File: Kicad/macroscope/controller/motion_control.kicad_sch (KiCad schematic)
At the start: 19 parts, among them J3 X stepper, J4 Y stepper, J5 Probe coil, M1 Stepper, M3 Stepper, U2 Coil driver

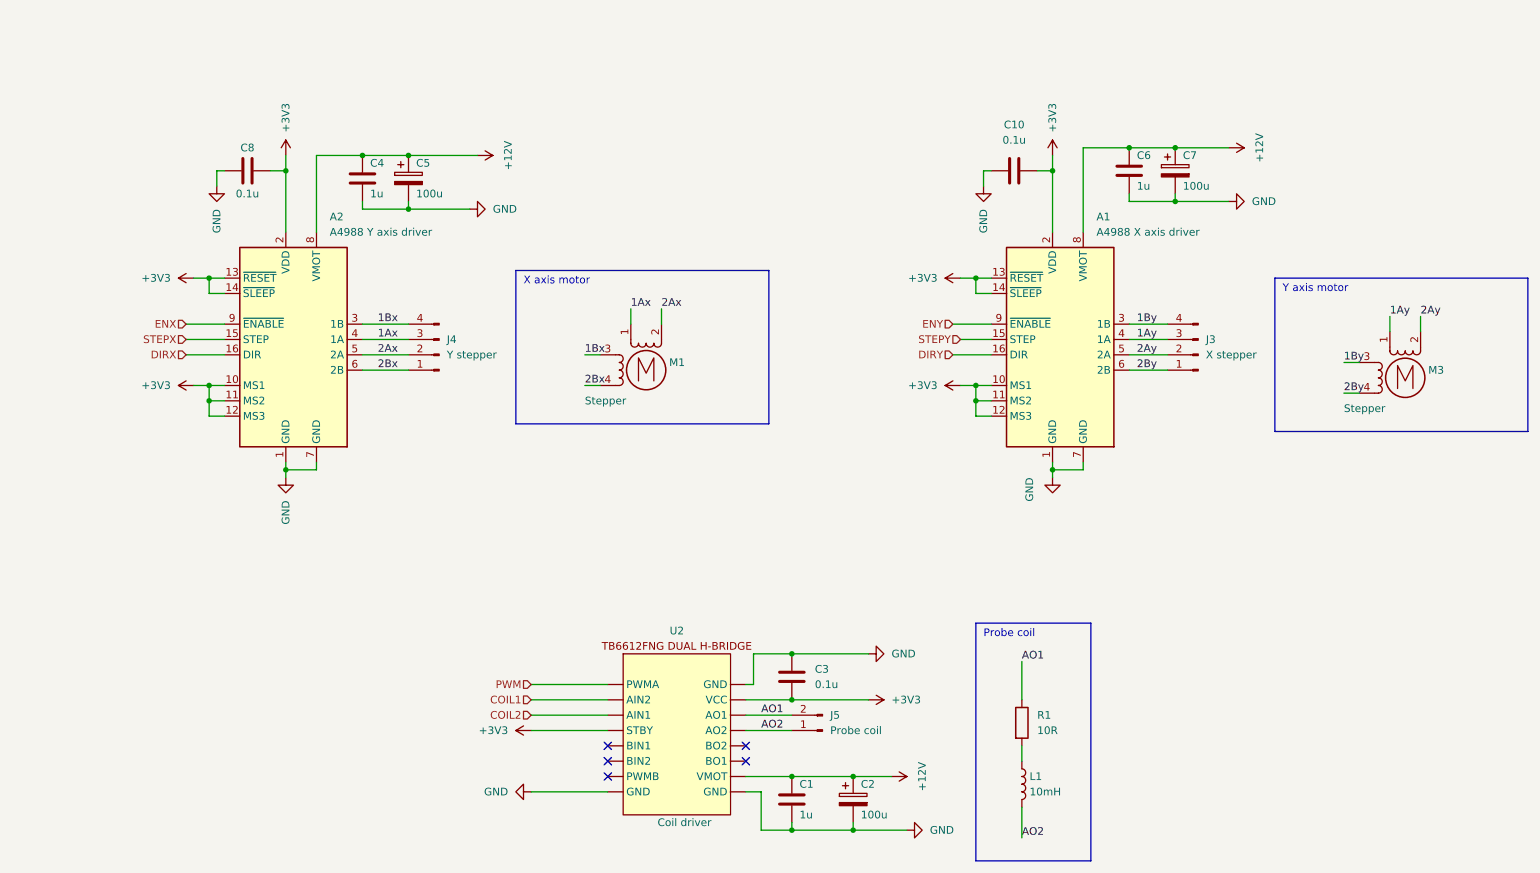
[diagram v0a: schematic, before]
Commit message: Update Kicad files
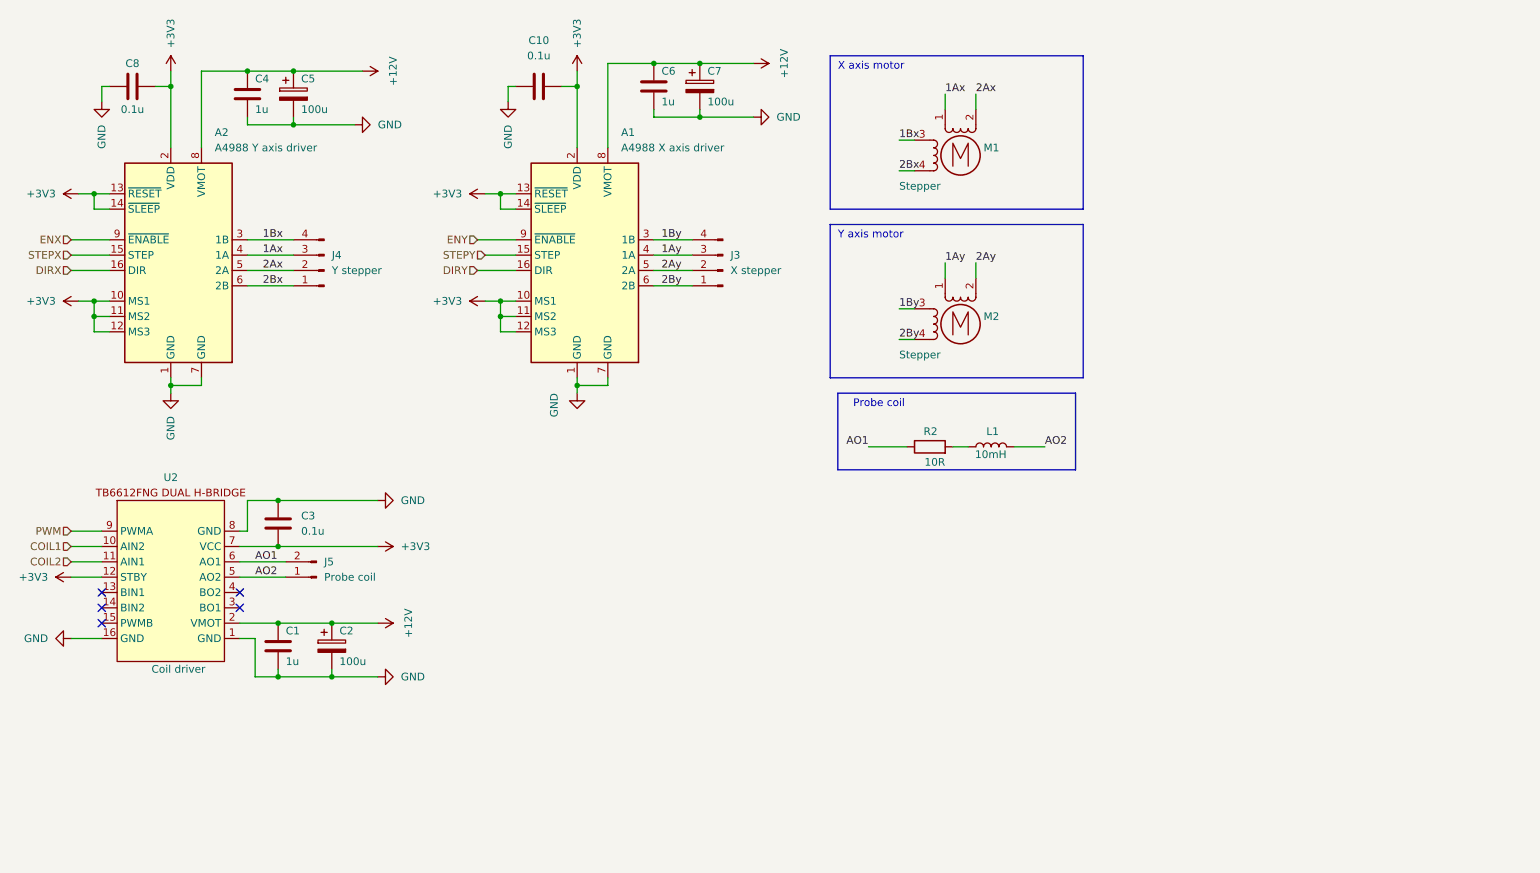
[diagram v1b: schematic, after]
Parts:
- C1, C10, C3, C4, C6, C8: footprint (none) -> Capacitor_SMD:C_1206_3216Metric
- C2, C5, C7: footprint (none) -> Capacitor_THT:CP_Radial_D6.3mm_P2.50mm
- J3, J4: footprint (none) -> Connector_PinHeader_2.54mm:PinHeader_1x04_P2.54mm_Vertical
- J5: footprint (none) -> Connector_Molex:Molex_KK-254_AE-6410-02A_1x02_P2.54mm_Vertical
- U2: footprint (none) -> Module:Pololu_Breakout-16_15.2x20.3mm
- renumbered M3 to M2, R1 to R2
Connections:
- net +12V: now also U2.2 (VMOT); no longer U2. (VMOT)
- net +3V3: now also U2.12 (STBY), U2.7 (VCC); no longer U2. (VMOT)
- net AO1: now also U2.6 (AO1); no longer U2. (VMOT)
- net AO2: now also U2.5 (AO2); no longer U2. (VMOT)
- net COIL1: now also U2.10 (AIN2); no longer U2. (VMOT)
- net COIL2: now also U2.11 (AIN1); no longer U2. (VMOT)
- net GND: now also U2.1 (GND), U2.16 (GND), U2.8 (GND); no longer U2. (VMOT)
- net PWM: now also U2.9 (PWMA); no longer U2. (VMOT)
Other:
- moved on the sheet: A1, A2, C1, C10, C2, C3, C4, C5, C6, C7, C8, J3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

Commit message: Add CAD
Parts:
- A1, A2: footprint Module:Pololu_Breakout-16_15.2x20.3mm -> Custom footprints:A4988_Pololu_Breakout-16_15.2x20.3mm
- U2: footprint Module:Pololu_Breakout-16_15.2x20.3mm -> Custom footprints:TB6612FNG_Pololu_Breakout-16_15.2x20.3mm
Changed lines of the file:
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@@
       (effects (font (size 1.27 1.27)))
     )
-    (property "Footprint" "Module:Pololu_Breakout-16_15.2x20.3mm" (at 41.91 106.68 0)
+    (property "Footprint" "Custom footprints:TB6612FNG_Pololu_Breakout-16_15.2x20.3mm" (at 41.91 106.68 0)
       (effects (font (size 1.27 1.27)) hide)
     )
@@
       (effects (font (size 1.27 1.27)) (justify left))
     )
-    (property "Footprint" "Module:Pololu_Breakout-16_15.2x20.3mm" (at 116.205 72.39 0)
+    (property "Footprint" "Custom footprints:A4988_Pololu_Breakout-16_15.2x20.3mm" (at 116.205 72.39 0)
       (effects (font (size 1.27 1.27)) (justify left) hide)
     )
@@
       (effects (font (size 1.27 1.27)) (justify left))
     )
-    (property "Footprint" "Module:Pololu_Breakout-16_15.2x20.3mm" (at 48.895 72.39 0)
+    (property "Footprint" "Custom footprints:A4988_Pololu_Breakout-16_15.2x20.3mm" (at 48.895 72.39 0)
       (effects (font (size 1.27 1.27)) (justify left) hide)
     )
